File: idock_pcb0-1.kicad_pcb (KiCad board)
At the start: 2 copper layers, 100 x 78 mm, 18 parts, among them J1 Barrel_Jack_Switch, J2 bluetooth-dock, J3 POWERLED, J4 PJRAN2X1U02, Q1 BC548, SW1 Reset, U1 ATmega32A-PU, Y1 8mhz

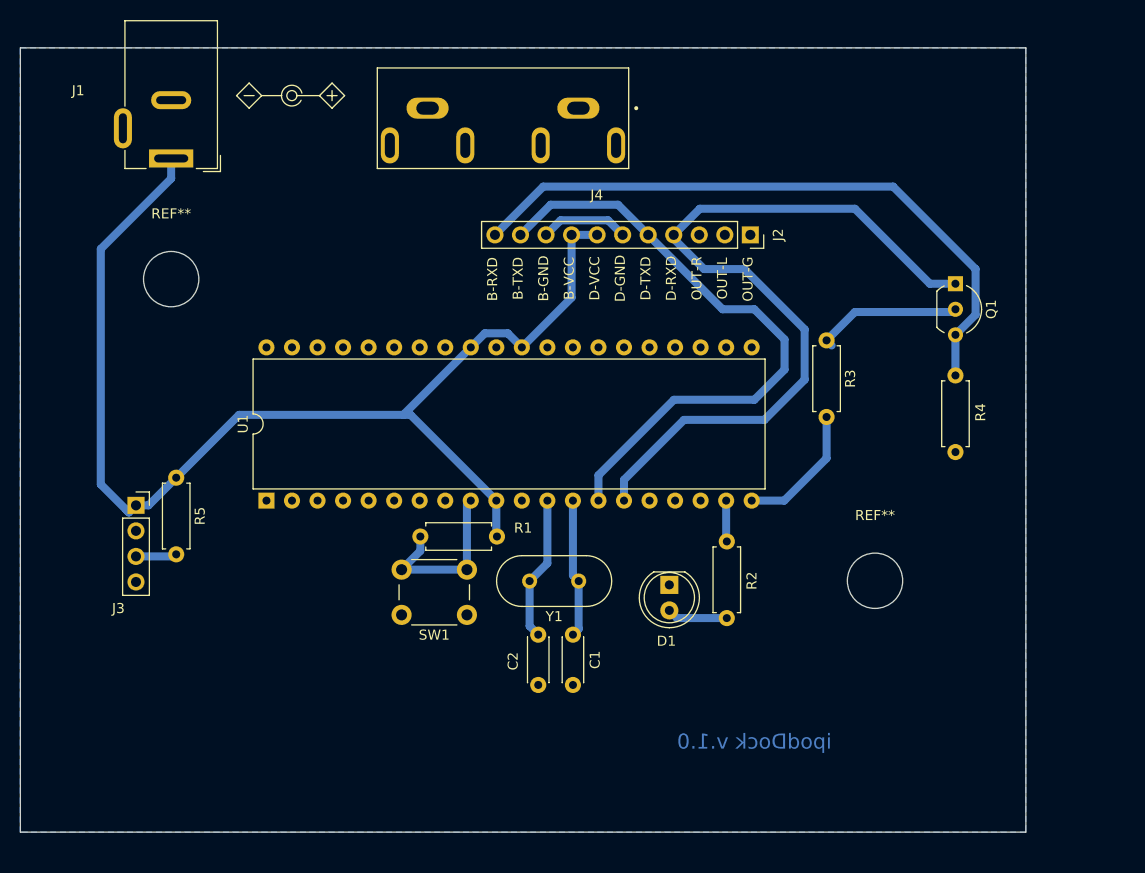
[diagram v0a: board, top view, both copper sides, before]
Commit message: printing tests
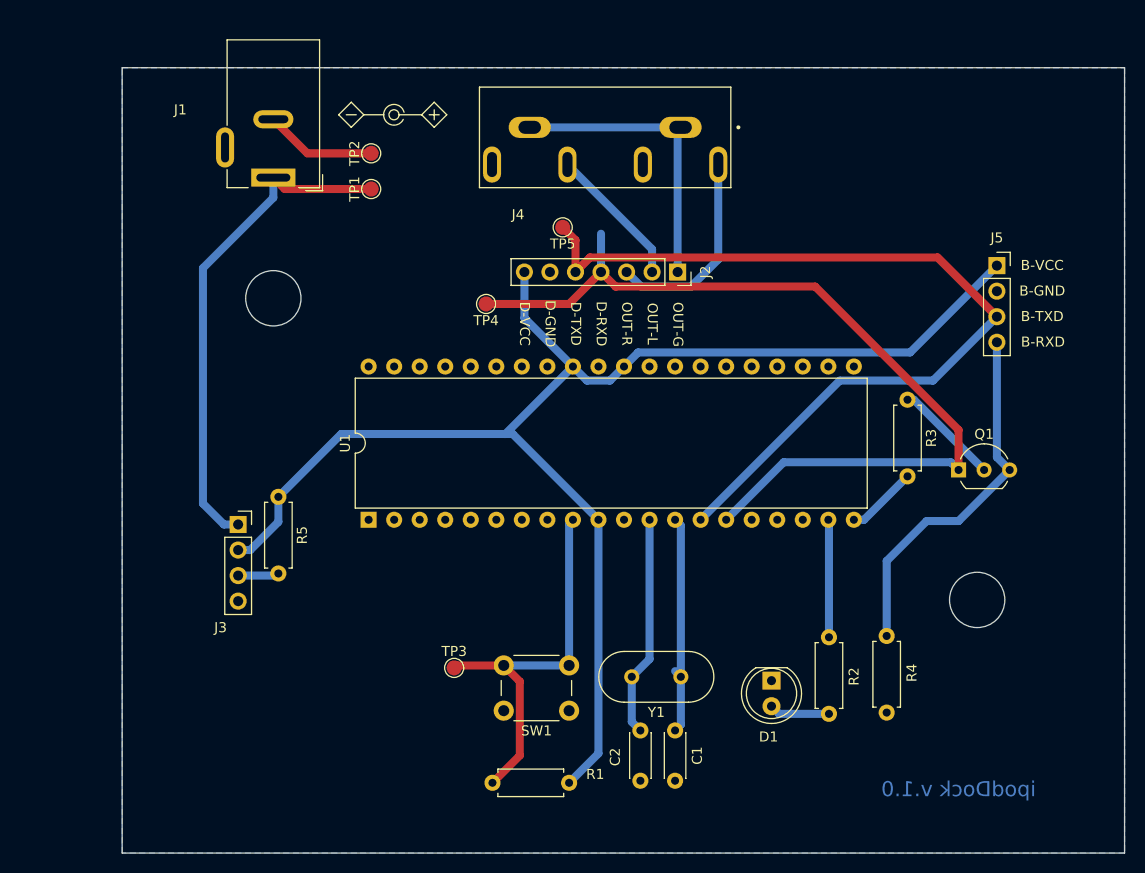
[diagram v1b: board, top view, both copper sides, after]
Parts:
- added J5: Bluetooth Module, Connector_PinSocket_2.54mm:PinSocket_1x04_P2.54mm_Vertical, F.Cu at (198.1, 73.7)
- added TP1: TestPoint, TestPoint:TestPoint_Pad_D1.5mm, F.Cu at (135.9, 66.0)
- added TP2: TestPoint, TestPoint:TestPoint_Pad_D1.5mm, F.Cu at (135.9, 62.5)
- added TP3: TestPoint, TestPoint:TestPoint_Pad_D1.5mm, F.Cu at (144.1, 113.7)
- added TP4: TestPoint, TestPoint:TestPoint_Pad_D1.5mm, F.Cu at (147.3, 77.5)
- added TP5: TestPoint, TestPoint:TestPoint_Pad_D1.5mm, F.Cu at (154.9, 69.8)
- J2: value bluetooth-dock -> dock; footprint Connector_PinSocket_2.54mm:PinSocket_1x11_P2.54mm_Vertical -> Connector_PinSocket_2.54mm:PinSocket_1x07_P2.54mm_Vertical
- moved R4 26.8 mm to (187.2, 118.1)
- moved R1 25.5 mm to (155.6, 125.1)
- moved Q1 18.5 mm to (194.3, 94.0), turned to 0 degrees
- moved C1 13.9 mm to (166.1, 119.9)
- moved C2 13.9 mm to (162.7, 119.9)
- moved D1 13.9 mm to (175.7, 114.9)
- moved SW1 13.9 mm to (155.6, 117.9)
- moved Y1 13.9 mm to (166.7, 114.6)
- moved R2 13.9 mm to (181.4, 118.2)
- moved ? 10.3 mm to (126.2, 76.9)
- moved ? 10.3 mm to (196.2, 106.9)
- moved J1 10.3 mm to (126.2, 64.9)
- moved J3 10.3 mm to (122.7, 99.4)
- moved J4 10.3 mm to (159.2, 59.9)
- moved R5 10.3 mm to (126.7, 96.7)
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- renumbered REF** to ?
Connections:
- J2 pad 5: Net-(J2-Pad10) -> Net-(J2-Pad5)
- Q1 pad 3: Net-(J2-Pad11) -> Net-(J5-Pad4)
- R4 pad 2: Net-(J2-Pad11) -> Net-(J5-Pad4)
- U1 pad 14: Net-(J2-Pad10) -> Net-(J2-Pad5)
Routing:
- net Net-(J2-Pad5): track 0.00 -> 87.8 mm
- net Net-(J2-Pad11): track 64.6 -> 0.00 mm
- net +5V: track 78.2 -> 141.3 mm
- net Net-(J2-Pad10): track 61.4 -> 0.00 mm
- net Net-(J5-Pad4): track 0.00 -> 36.7 mm
- net Net-(J2-Pad1): track 0.00 -> 29.5 mm
- net Net-(R1-Pad2): track 17.6 -> 39.6 mm
- net Net-(J2-Pad3): track 0.00 -> 20.3 mm
- net Net-(J2-Pad2): track 0.00 -> 14.2 mm
- net Net-(J1-Pad1): track 39.7 -> 49.9 mm
- net Net-(J2-Pad4): track 78.5 -> 88.4 mm
- net Net-(C1-Pad1): track 13.8 -> 22.2 mm
- net Net-(R2-Pad2): track 4.09 -> 11.8 mm
- net Net-(C2-Pad1): track 14.4 -> 22.0 mm
- net Net-(R3-Pad2): track 13.3 -> 7.12 mm
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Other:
- board size 100 x 78 mm -> 99.7 x 78.1 mm
